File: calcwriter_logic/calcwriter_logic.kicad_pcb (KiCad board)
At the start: 4 copper layers, 33 x 62.8 mm, 46 parts, among them CON1 FH12-40S-0.5SH_55_, IC1 MAX335CWG_T, IC2 MAX335CWG_T, IC3 MAX335CWG_T, IC4 MAX335CWG_T, J1 USB_C_Receptacle_USB2.0_14P, U1 ATmega32U4-A, U2 ME6211C15M5G-N, Y1 16MHz

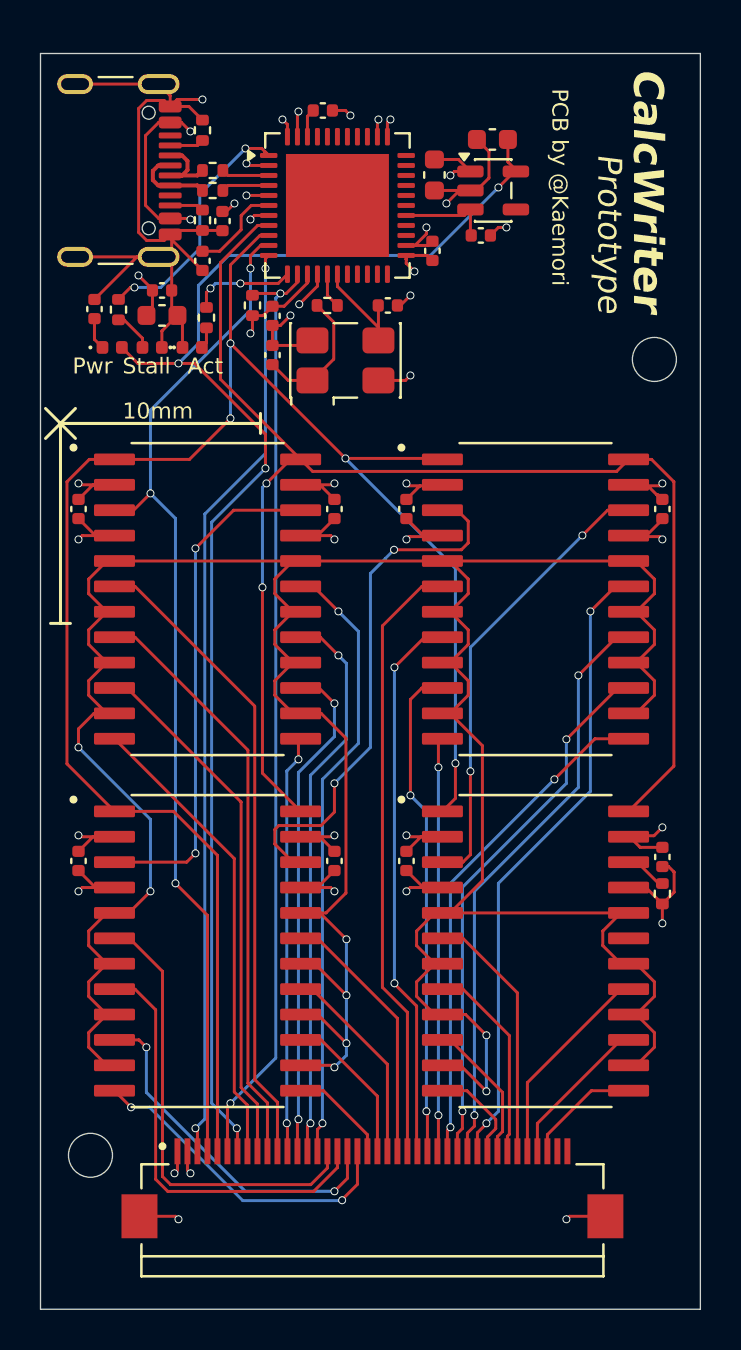
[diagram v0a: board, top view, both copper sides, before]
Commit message: did another thing AAAAAAAAAAAAAAAAAAA
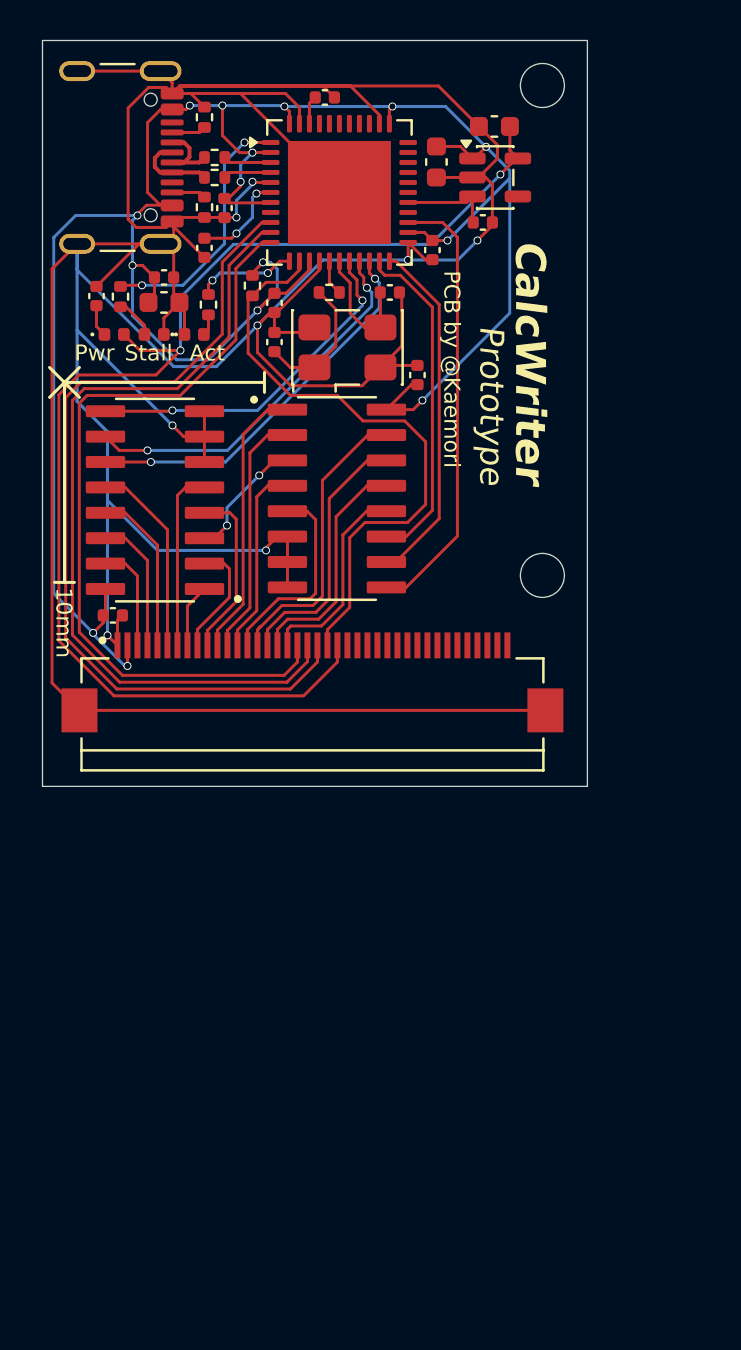
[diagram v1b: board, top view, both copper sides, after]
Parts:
- removed C1, C2, C3, C4, C5, C6, C7, C8: 100nF, Capacitor_SMD:C_0402_1005Metric
- removed EXPLORPHEUS, HACKCLUB: LOGO, LOGO
- removed IC1, IC2, IC3, IC4: MAX335CWG_T, MAX335CWG_T:SOIC127P1032X265-24N
- removed R1: 10k, Resistor_SMD:R_0402_1005Metric
- removed SCREW2: MountingHole_2.2mm_M2, MountingHole:MountingHole_2.2mm_M2
- added G***: LOGO, LOGO, B.Cu at (130.7, 61.0)
- added G***: LOGO, LOGO, B.Cu at (121.5, 76.5)
- added MUX_C1: 100nF, Capacitor_SMD:C_0402_1005Metric, F.Cu at (116.0, 85.5)
- added MUX_C2: 100nF, Capacitor_SMD:C_0402_1005Metric, F.Cu at (131.2, 73.5)
- added SCREW1: MountingHole_2.2mm_M2, MountingHole:MountingHole_2.2mm_M2, F.Cu at (137.5, 59.0)
- added U3: SN74LV4051ADR, SN74LV4051ADR:SOIC127P600X175-16N, F.Cu at (118.1, 79.7)
- added U4: SN74LV4051ADR, SN74LV4051ADR:SOIC127P600X175-16N, F.Cu at (127.2, 79.7)
- U1: value ATmega32U4-A -> ATmega32U4-MU
- moved CON1 25.5 mm to (126.0, 87.0)
- moved SCREW1 12.2 mm to (137.5, 83.5)
- moved RST_PU1 0.99 mm to (123.0, 69.0), turned to 90 degrees
- moved CALC_PWR_R1 0.66 mm to (134.5, 65.8)
- moved CALC_PWR_R2 0.66 mm to (115.2, 69.5)
- moved OSC_R1 0.66 mm to (126.8, 69.3)
- moved PWR_C1 0.66 mm to (118.6, 69.8)
- moved CALC_PWR_C2 0.66 mm to (135.1, 61.0)
- moved LED_R2 0.66 mm to (120.8, 70.0)
- moved OSC_C1 0.66 mm to (129.9, 69.3)
- moved OSC_C2 0.66 mm to (124.1, 71.8)
- moved PWR_C2 0.66 mm to (118.6, 68.6)
- moved U1 0.66 mm to (127.3, 64.3)
- moved VCC_C3 0.66 mm to (121.6, 65.1)
- moved Y1 0.66 mm to (127.8, 72.1)
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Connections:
- CON1 pad 10: /CONN_3 -> /A7
- CON1 pad 11: /CONN_4 -> /B4
- CON1 pad 12: /CONN_5 -> /B6
- CON1 pad 13: /CONN_6 -> /B7
- CON1 pad 14: /CONN_7 -> /B5
- CON1 pad 15: /CONN_8 -> /B2
- CON1 pad 16: /CONN_9 -> /B1
- CON1 pad 17: /CONN_10 -> /B0
- CON1 pad 18: /CONN_11 -> /B3
- CON1 pad 19: /CONN_12 -> ISP_MISO
- CON1 pad 20: /CONN_13 -> ISP_MOSI
- CON1 pad 21: /CONN_14 -> ISP_SCK
- CON1 pad 22: /CONN_15 -> ISP_RST
- CON1 pad 23: /CONN_16 -> +1V5
- CON1 pad 24: /CONN_17 -> unconnected-(CON1-Pad24)
- CON1 pad 25: /CONN_18 -> unconnected-(CON1-Pad25)
- CON1 pad 26: /CONN_19 -> unconnected-(CON1-Pad26)
- CON1 pad 27: /CONN_20 -> unconnected-(CON1-Pad27)
- CON1 pad 28: /CONN_21 -> unconnected-(CON1-Pad28)
- CON1 pad 29: /CONN_22 -> unconnected-(CON1-Pad29)
- CON1 pad 3: ISP_MISO -> /A2
- CON1 pad 30: /CONN_23 -> unconnected-(CON1-Pad30)
- CON1 pad 31: /CONN_24 -> unconnected-(CON1-Pad31)
- CON1 pad 32: /CONN_25 -> unconnected-(CON1-Pad32)
- CON1 pad 33: /CONN_26 -> unconnected-(CON1-Pad33)
- CON1 pad 34: /CONN_27 -> unconnected-(CON1-Pad34)
- CON1 pad 35: /CONN_28 -> unconnected-(CON1-Pad35)
- CON1 pad 36: /CONN_29 -> unconnected-(CON1-Pad36)
- CON1 pad 37: /CONN_30 -> unconnected-(CON1-Pad37)
- CON1 pad 38: /CONN_31 -> unconnected-(CON1-Pad38)
- CON1 pad 4: ISP_MOSI -> /A1
- CON1 pad 5: CLK -> /A0
- CON1 pad 6: ISP_RST -> /A3
- CON1 pad 7: +1V5 -> /A5
- CON1 pad 8: /CONN_1 -> /A4
- CON1 pad 9: /CONN_2 -> /A6
- U1 pad 18: unconnected-(U1-PD0-Pad18) -> CH1C
- U1 pad 19: unconnected-(U1-PD1-Pad19) -> CH1B
- U1 pad 20: unconnected-(U1-PD2-Pad20) -> CH1A
- U1 pad 21: unconnected-(U1-PD3-Pad21) -> CH2A
- U1 pad 22: unconnected-(U1-PD5-Pad22) -> CH2B
- U1 pad 25: unconnected-(U1-PD4-Pad25) -> CH2C
- U1 pad 45: (no net) -> GND
- U1 pad 8: CS -> unconnected-(U1-PB0-Pad8)
- U1 pad 9: CLK -> ISP_SCK
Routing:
- net CONN_BUS: track 161.4 -> 0.00 mm, vias 8 -> 0
- net GND: track 90.1 -> 248.0 mm, vias 23 -> 8
- net CLK: track 91.1 -> 0.00 mm, vias 4 -> 0
- net CS: track 70.7 -> 0.00 mm, vias 2 -> 0
- net VBUS: track 51.6 -> 119.4 mm, vias 20 -> 15
- net ISP_SCK: track 0.00 -> 43.0 mm
- net /CONN_4: track 32.2 -> 0.00 mm
- net /CONN_24: track 31.1 -> 0.00 mm, vias 2 -> 0
- net /CONN_17: track 30.6 -> 0.00 mm
- net /CONN_8: track 30.0 -> 0.00 mm, vias 2 -> 0
- net /CONN_3: track 29.5 -> 0.00 mm
- net /CONN_23: track 28.8 -> 0.00 mm, vias 2 -> 0
- net /CONN_7: track 28.0 -> 0.00 mm, vias 2 -> 0
- net /CONN_18: track 26.8 -> 0.00 mm, vias 2 -> 0
- net /CONN_22: track 26.5 -> 0.00 mm, vias 2 -> 0
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- removed copper zone on In1.Cu, net GND
- removed copper zone on In2.Cu, net VBUS
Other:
- board size 33 x 62.8 mm -> 27.2 x 37.3 mm
- copper layers 4 -> 2
